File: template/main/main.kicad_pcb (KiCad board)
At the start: 2 copper layers, 99.1 x 99.1 mm, 8 parts, among them J2 PinHeader_01x05_P2.54_THT_ang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

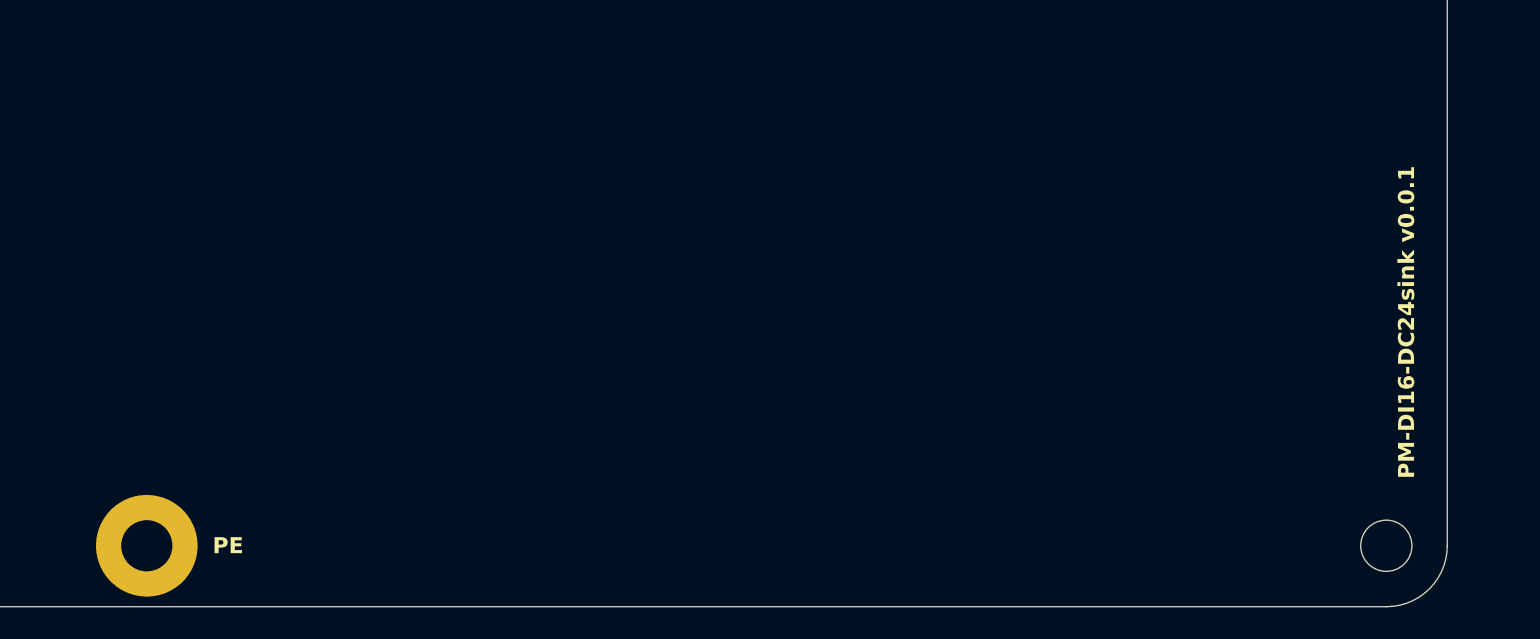
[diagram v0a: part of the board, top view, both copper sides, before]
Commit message: PM-PS
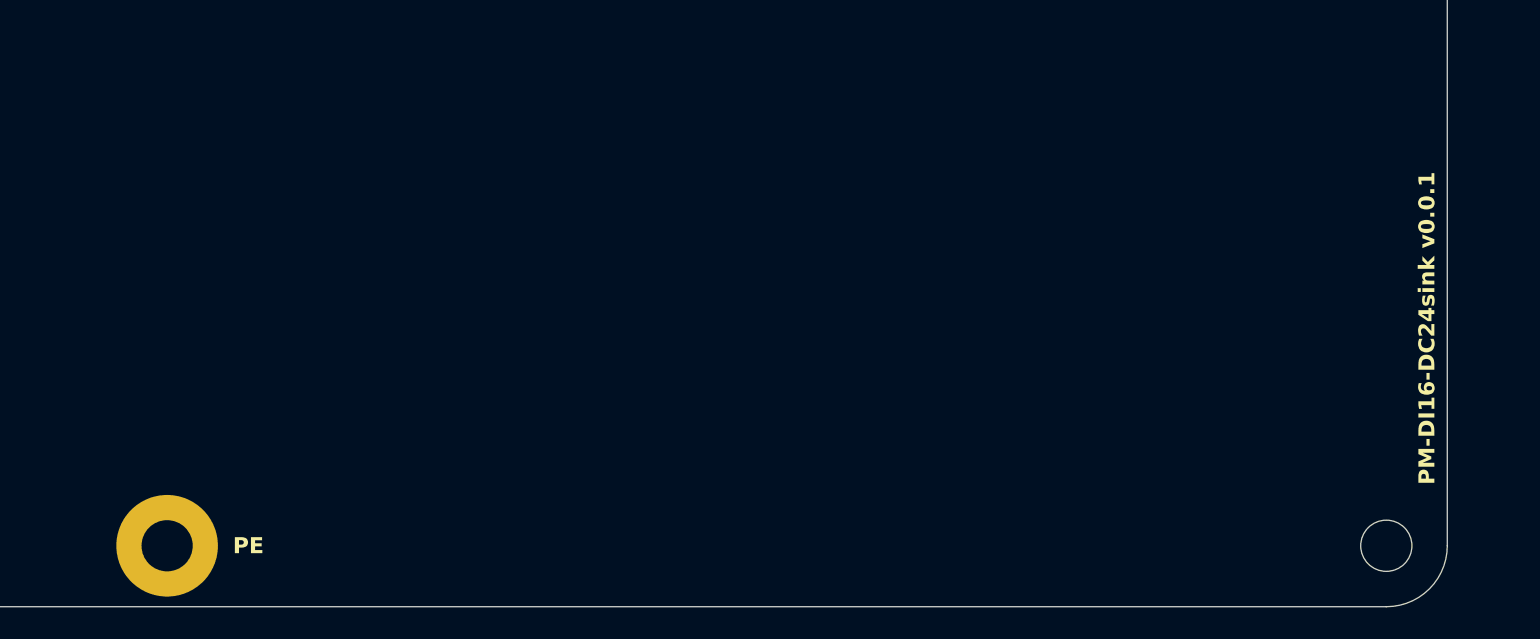
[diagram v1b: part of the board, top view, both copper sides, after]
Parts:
- moved PE1 1.27 mm to (44.5, 146.1)
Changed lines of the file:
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@@
 	(footprint "kicad_inventree_lib:PE"
 		(layer "F.Cu")
-		(at 43.18 146.05)
+		(at 44.45 146.05)
 		(property "Reference" "PE1"
 			(at 0 -6.5 0)
@@
 	)
 	(gr_text "PE"
-		(at 48.26 146.05 -0)
+		(at 49.53 146.05 -0)
 		(layer "B.SilkS" knockout)
 		(effects
@@
 	)
 	(gr_text "PE"
-		(at 48.26 146.05 0)
+		(at 49.53 146.05 0)
 		(layer "F.SilkS" knockout)
 		(effects
@@
 	)
 	(gr_text "PM-DI16-DC24sink v0.0.1"
-		(at 121.92 132.08 90)
+		(at 123.19 142.24 90)
 		(layer "F.SilkS" knockout)
 		(effects
@@
 				(bold yes)
 			)
-		)
-	)
+			(justify left)
+		)
+	)
